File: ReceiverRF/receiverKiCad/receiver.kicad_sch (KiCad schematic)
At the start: 23 parts, among them J2 Conn_01x05_Socket, U1 STM32F103RET6, Y1 YG8M000000S418

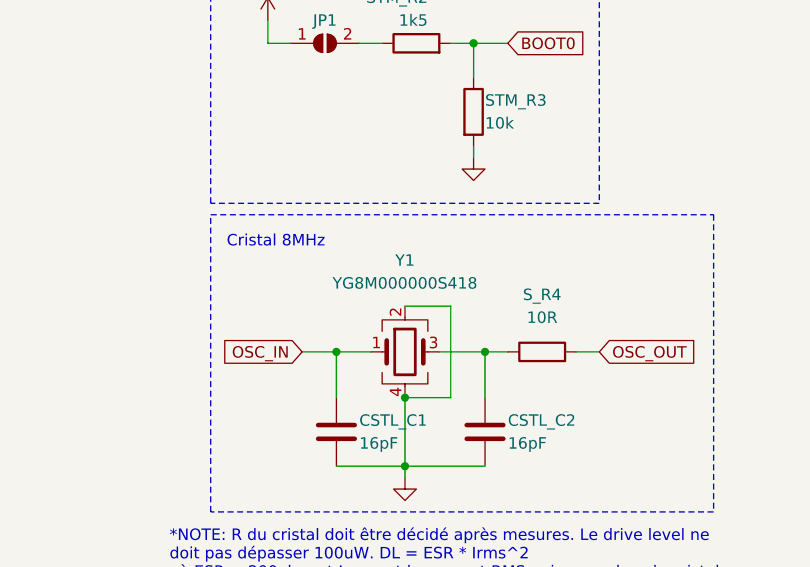
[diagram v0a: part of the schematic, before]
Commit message: changement cristal
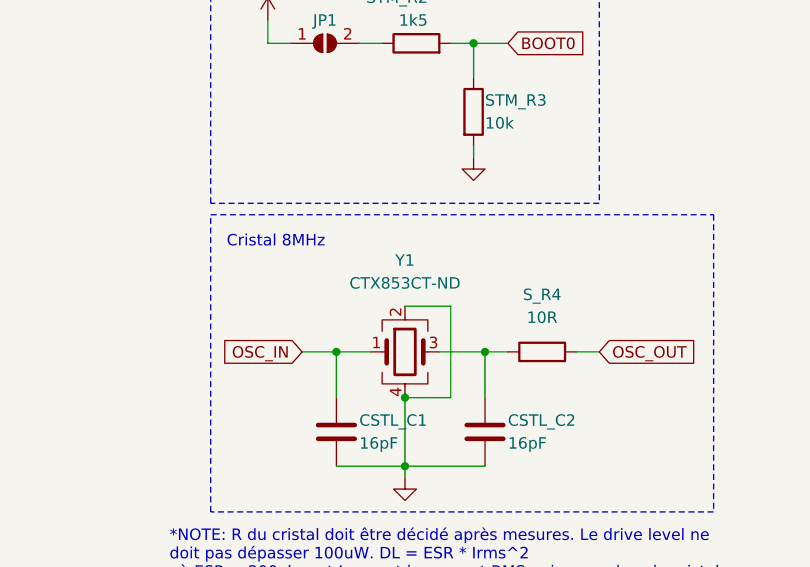
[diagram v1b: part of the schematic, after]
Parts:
- Y1: value YG8M000000S418 -> CTX853CT-ND; Digikey 3372-YG8M000000S418TR-ND -> CTX853CT-ND
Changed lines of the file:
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@@
 			)
 		)
-		(property "Value" "YG8M000000S418"
+		(property "Value" "CTX853CT-ND"
 			(at 238.76 118.11 0)
 			(effects
@@
 			)
 		)
-		(property "Datasheet" "https://www.digikey.ca/en/products/detail/nextgen-components/YG8M000000S416/17289334"
+		(property "Datasheet" "https://www.digikey.ca/en/products/detail/cts-frequency-controls/406C35D08M00000/2292774"
 			(at 238.76 125.73 0)
 			(effects
@@
 			)
 		)
-		(property "Description" "YG8M000000S416"
+		(property "Description" "406C35D08M00000"
 			(at 238.76 125.73 0)
 			(effects
@@
 			)
 		)
-		(property "Digikey" "  3372-YG8M000000S418TR-ND"
+		(property "Digikey" "CTX853CT-ND"
 			(at 238.76 125.73 0)
 			(effects
